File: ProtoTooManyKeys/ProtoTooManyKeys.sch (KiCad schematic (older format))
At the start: 74 parts, among them J1 54104-3031_Oled, J2 AVR-ISP-6, SW1 SW_Push, U1 PRTR5V0U2X, U2 AT90USB1286-AU, U3 PCA9306TDCURQ1, U4 AZ1117CH-3.3TRG1, Y1 16MHz

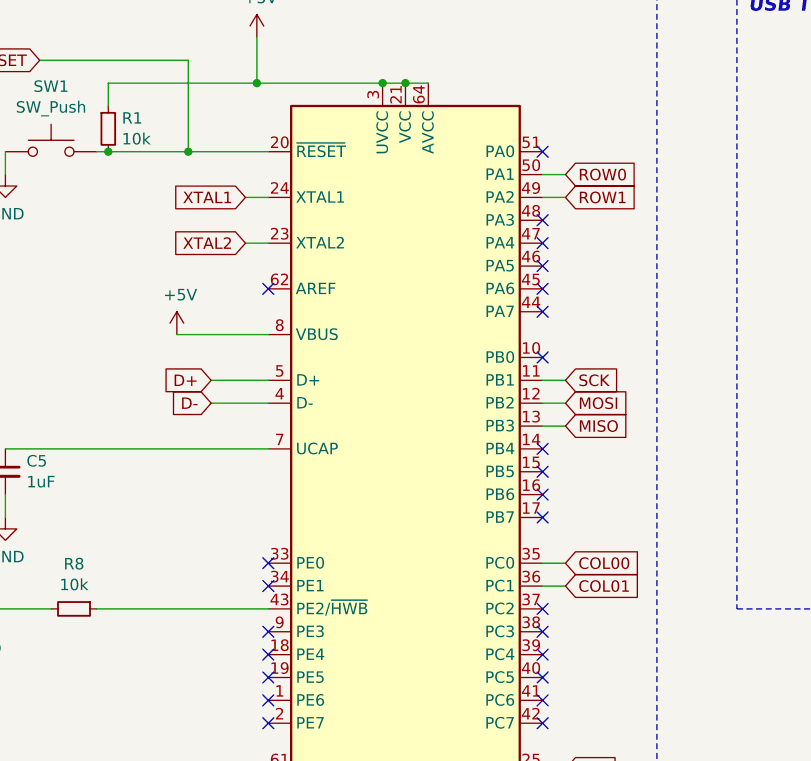
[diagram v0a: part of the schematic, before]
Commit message: Routing finished
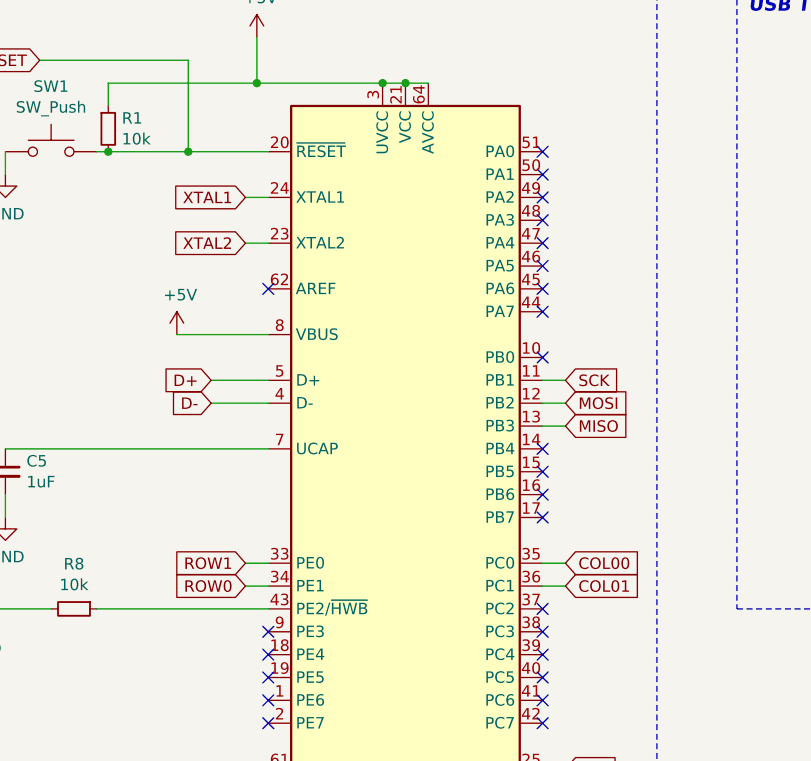
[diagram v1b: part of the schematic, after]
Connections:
- net ROW0: now also U2.34 (PE1); no longer U2.50 (PA1)
- net ROW1: now also U2.33 (PE0); no longer U2.49 (PA2)
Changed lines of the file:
@@
 Text GLabel 4200 4200 2    50   Input ~ 0
 SDA
-Text GLabel 4200 1600 2    50   Input ~ 0
+Text GLabel 2800 3200 0    50   Input ~ 0
 ROW1
-Text GLabel 4200 1500 2    50   Input ~ 0
+Text GLabel 2800 3300 0    50   Input ~ 0
 ROW0
 Text GLabel 4200 3200 2    50   Input ~ 0
@@
 $EndComp
 Wire Wire Line
-	4200 1500 4100 1500
-Wire Wire Line
-	4200 1600 4100 1600
+	2800 3300 2900 3300
+Wire Wire Line
+	2800 3200 2900 3200
 Text GLabel 10350 2400 0    50   Input ~ 0
 RESET
@@
 NoConn ~ 4100 3800
 NoConn ~ 4100 3900
-NoConn ~ 2900 3200
-NoConn ~ 2900 3300
 NoConn ~ 2900 3800
 NoConn ~ 2900 3900
@@
 	1    0    0    -1
 $EndComp
+NoConn ~ 4100 1500
+NoConn ~ 4100 1600
 $EndSCHEMATC
